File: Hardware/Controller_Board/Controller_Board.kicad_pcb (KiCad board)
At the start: 8 copper layers, 211 parts, among them J103 USB_C_USB2.0, Q1 DMN2400UFB-7, SW1 Reset, U1 TPS82084, U10 FT232H, U11 93LC56B, U12 USB2512B, U14 RJ45, U15 TPD4E02B04, U16 RJ45, U17 RJ45, U18 TPD4E02B04, U19 TPD4E02B04, U2 LT8645S, U20 TPD4E02B04, U21 TPD4E02B04, U22 RJ45, U23 TPD4E02B04, U24 TPD4E02B04, U25 RJ45, U26 TPD4E02B04, U27 TPD4E02B04, U28 RJ45, U29 TPD4E02B04, U3 TPS82084, U30 TPD4E02B04, U31 RJ45, U32 TPD4E02B04, U33 TPD4E02B04, U34 RJ45, U37 RJ45, U39 TPD4E02B04, U4 TPS82084, U5 XT30, U501 TPD4E02B04, U6 XC7A35T-CPG236, U7 IS25LP256D, U8 FT232H, U9 93LC56B, Y1 12MHz, Y2 12MHz, Y3 24MHz, Y301 12MHz

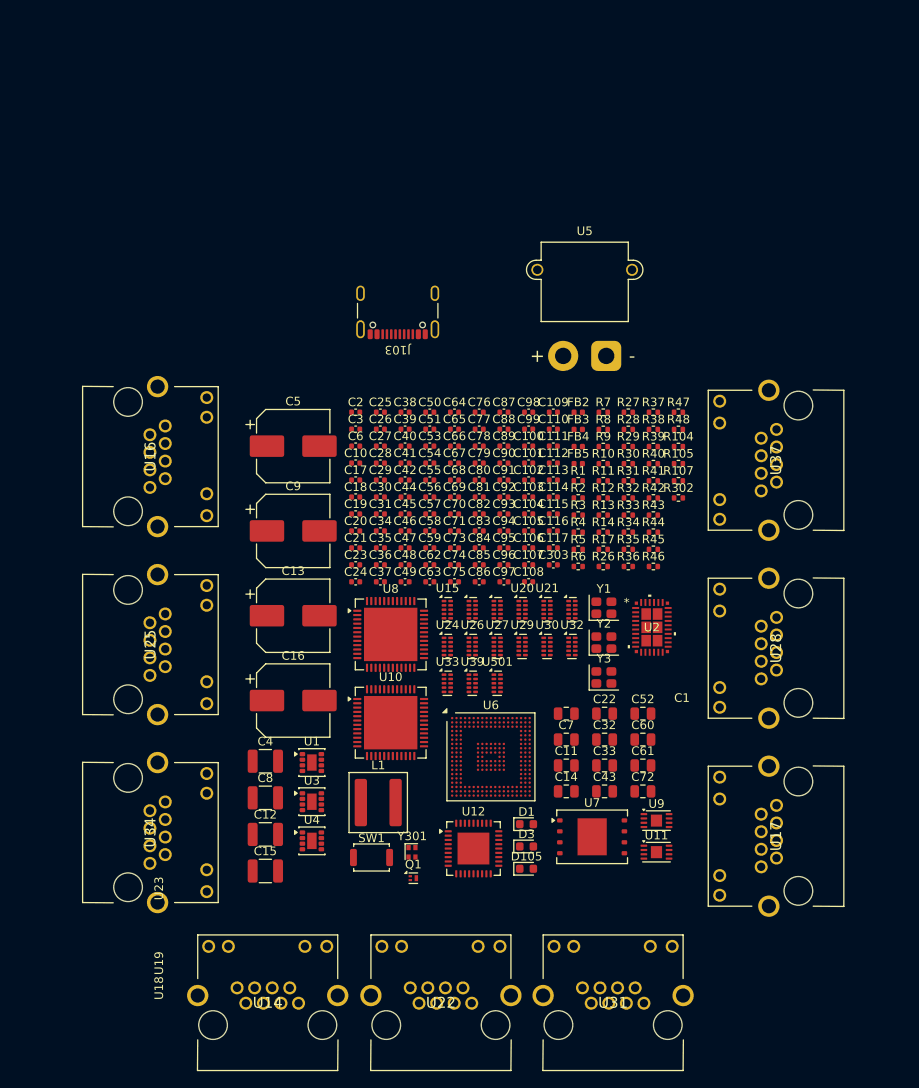
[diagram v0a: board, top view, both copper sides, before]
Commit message: Finished the schematic review
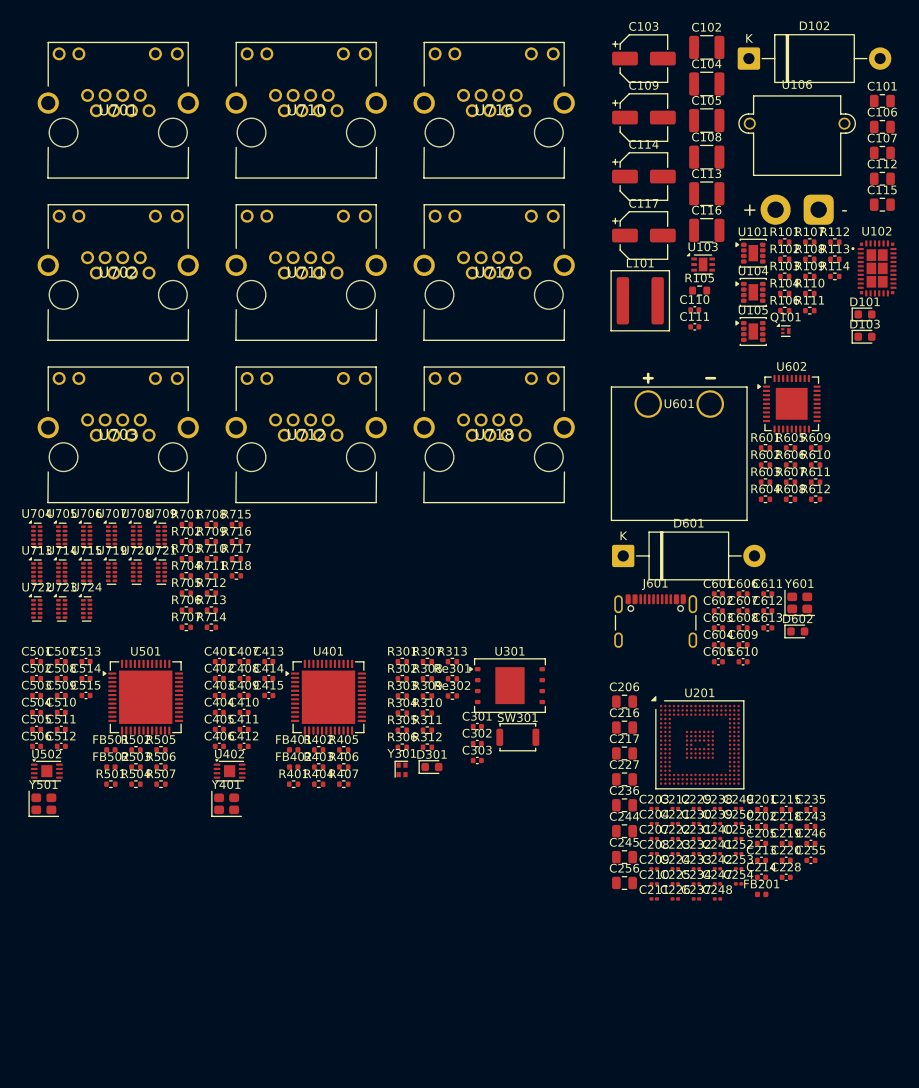
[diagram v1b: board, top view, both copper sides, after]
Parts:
- removed C1, C11, C14, C22, C32, C33, C43, C52, C60, C61, C7, C72: 10u, Capacitor_SMD:C_0805_2012Metric
- removed C10, C17, C19, C20, C23, C24, C25, C26, C27, C28, C37, C38, C39, C40, C41, C42, C45, C46, C47, C48, C49, C50, C53, C54, C55, C56, C57, C58, C63, C64, C65, C66, C67, C68, C69, C70, C73, C76, C77, C78, C79, C80, C81, C82, C84, C86, C87, C91, C92, C93, C94, C95, C96, C97, C99: 100n, Capacitor_SMD:C_0402_1005Metric
- removed C100, C75, C83, C85, C90, C98: 4u7, Capacitor_SMD:C_0402_1005Metric
- removed C12, C15, C4, C8: 22u, Capacitor_SMD:C_1210_3225Metric
- removed C13, C16, C5, C9: 100u, Capacitor_SMD:CP_Elec_8x6.5
- removed C18, C88, C89: 10p, Capacitor_SMD:C_0402_1005Metric
- removed C2, C3: 470n, Capacitor_SMD:C_0402_1005Metric
- removed C21, C29, C30, C31, C34, C35, C36, C44, C51, C59, C62, C71, C74: 1u, Capacitor_SMD:C_0402_1005Metric
- removed C6: 2.2p, Capacitor_SMD:C_0402_1005Metric
- removed D1, D105, D3: LED, LED_SMD:LED_0603_1608Metric
- removed FB2, FB3, FB4, FB5: 600R, Inductor_SMD:L_0402_1005Metric
- removed J103: USB_C_USB2.0, Connector_USB:USB_C_Receptacle_GCT_USB4105-xx-A_16P_TopMnt_Horizontal
- removed L1: 2u2, Inductor_SMD:L_Coilcraft_XAL6030-XXX
- removed Q1: DMN2400UFB-7, Package_DFN_QFN:Diodes_DFN1006-3
- removed R1: 1Meg, Resistor_SMD:R_0402_1005Metric
- removed R10, R2, R7: 499k, Resistor_SMD:R_0402_1005Metric
- removed R11: 156.3k, Resistor_SMD:R_0402_1005Metric
- removed R12, R5, R9: 50k, Resistor_SMD:R_0402_1005Metric
- removed R13: 280R, Resistor_SMD:R_0402_1005Metric
- removed R14, R17: 200R, Resistor_SMD:R_0402_1005Metric
- removed R26, R33, R48: 1k, Resistor_SMD:R_0402_1005Metric
- removed R27, R34, R41: 12k, Resistor_SMD:R_0402_1005Metric
- removed R28, R29, R30, R35, R36, R37: 10k, Resistor_SMD:R_0402_1005Metric
- removed R3: 12.5k, Resistor_SMD:R_0402_1005Metric
- removed R31, R38: 2k2, Resistor_SMD:R_0402_1005Metric
- removed R32, R39, R40: 22R, Resistor_SMD:R_0402_1005Metric
- removed R4: 243k, Resistor_SMD:R_0402_1005Metric
- removed R42, R43, R44, R45, R46, R47: 100k, Resistor_SMD:R_0402_1005Metric
- removed R6: 41.2k, Resistor_SMD:R_0402_1005Metric
- removed R8: 62.5k, Resistor_SMD:R_0402_1005Metric
- removed SW1: Reset, Button_Switch_SMD:SW_Push_SPST_NO_Alps_SKRK
- removed U1, U3, U4: TPS82084, Package_LGA:Texas_SIL0008C_MicroSiP-8-1EP_2.8x3mm_P0.65mm_EP1.1x1.9mm
- removed U10, U8: FT232H, Package_DFN_QFN:QFN-48-1EP_8x8mm_P0.5mm_EP6.2x6.2mm
- removed U11, U9: 93LC56B, Package_DFN_QFN:TDFN-8-1EP_3x2mm_P0.5mm_EP1.3x1.4mm
- removed U12: USB2512B, Package_DFN_QFN:QFN-36-1EP_6x6mm_P0.5mm_EP3.7x3.7mm
- removed U14, U16, U17, U22, U25, U28, U31, U34, U37: RJ45, Custom_VoxLink_Footprints:TE_RJ45
- removed U15, U18, U19, U20, U21, U23, U24, U26, U27, U29, U30, U32, U33, U39: TPD4E02B04, Package_SON:USON-10_2.5x1.0mm_P0.5mm
- removed U2: LT8645S, Custom_VoxLink_Footprints:LT8645S
- removed U5: XT30, Connector_AMASS:AMASS_XT30PW-M_1x02_P2.50mm_Horizontal
- removed U6: XC7A35T-CPG236, Package_BGA:Xilinx_CPG236
- removed U7: IS25LP256D, Package_SON:WSON-8-1EP_8x6mm_P1.27mm_EP3.4x4.3mm
- removed Y1, Y2: 12MHz, Crystal:Crystal_SMD_2520-4Pin_2.5x2.0mm
- removed Y3: 24MHz, Crystal:Crystal_SMD_2520-4Pin_2.5x2.0mm
- added C201: 100n, Capacitor_SMD:C_0402_1005Metric, F.Cu at (160.2, 121.0)
- added C202: 10p, Capacitor_SMD:C_0402_1005Metric, F.Cu at (160.2, 122.9)
- added C203: 100n, Capacitor_SMD:C_0201_0603Metric, F.Cu at (147.8, 120.8)
- added C204: 100n, Capacitor_SMD:C_0201_0603Metric, F.Cu at (147.8, 122.6)
- added C205: 1u, Capacitor_SMD:C_0402_1005Metric, F.Cu at (160.2, 124.9)
- added C206: 10u, Capacitor_SMD:C_0805_2012Metric, F.Cu at (144.3, 108.4)
- added C207: 100n, Capacitor_SMD:C_0201_0603Metric, F.Cu at (147.8, 124.3)
- added C208: 100n, Capacitor_SMD:C_0201_0603Metric, F.Cu at (147.8, 126.1)
- added C209: 100n, Capacitor_SMD:C_0201_0603Metric, F.Cu at (147.8, 127.8)
- added C210: 100n, Capacitor_SMD:C_0201_0603Metric, F.Cu at (147.8, 129.6)
- added C211: 100n, Capacitor_SMD:C_0201_0603Metric, F.Cu at (147.8, 131.3)
- added C212: 100n, Capacitor_SMD:C_0201_0603Metric, F.Cu at (150.2, 120.8)
- added C213: 1u, Capacitor_SMD:C_0402_1005Metric, F.Cu at (160.2, 126.9)
- added C214: 1u, Capacitor_SMD:C_0402_1005Metric, F.Cu at (160.2, 128.8)
- added C215: 1u, Capacitor_SMD:C_0402_1005Metric, F.Cu at (163.1, 121.0)
- added C216: 10u, Capacitor_SMD:C_0805_2012Metric, F.Cu at (144.3, 111.4)
- added C217: 10u, Capacitor_SMD:C_0805_2012Metric, F.Cu at (144.3, 114.5)
- added C218: 1u, Capacitor_SMD:C_0402_1005Metric, F.Cu at (163.1, 122.9)
- added C219: 1u, Capacitor_SMD:C_0402_1005Metric, F.Cu at (163.1, 124.9)
- added C220: 1u, Capacitor_SMD:C_0402_1005Metric, F.Cu at (163.1, 126.9)
- added C221: 100n, Capacitor_SMD:C_0201_0603Metric, F.Cu at (150.2, 122.6)
- added C222: 100n, Capacitor_SMD:C_0201_0603Metric, F.Cu at (150.2, 124.3)
- added C223: 100n, Capacitor_SMD:C_0201_0603Metric, F.Cu at (150.2, 126.1)
- added C224: 100n, Capacitor_SMD:C_0201_0603Metric, F.Cu at (150.2, 127.8)
- added C225: 100n, Capacitor_SMD:C_0201_0603Metric, F.Cu at (150.2, 129.6)
- added C226: 100n, Capacitor_SMD:C_0201_0603Metric, F.Cu at (150.2, 131.3)
- added C227: 10u, Capacitor_SMD:C_0805_2012Metric, F.Cu at (144.3, 117.5)
- added C228: 1u, Capacitor_SMD:C_0402_1005Metric, F.Cu at (163.1, 128.8)
- added C229: 100n, Capacitor_SMD:C_0201_0603Metric, F.Cu at (152.7, 120.8)
- added C230: 100n, Capacitor_SMD:C_0201_0603Metric, F.Cu at (152.7, 122.6)
- added C231: 100n, Capacitor_SMD:C_0201_0603Metric, F.Cu at (152.7, 124.3)
- added C232: 100n, Capacitor_SMD:C_0201_0603Metric, F.Cu at (152.7, 126.1)
- added C233: 100n, Capacitor_SMD:C_0201_0603Metric, F.Cu at (152.7, 127.8)
- added C234: 100n, Capacitor_SMD:C_0201_0603Metric, F.Cu at (152.7, 129.6)
- added C235: 1u, Capacitor_SMD:C_0402_1005Metric, F.Cu at (166.0, 121.0)
- added C236: 10u, Capacitor_SMD:C_0805_2012Metric, F.Cu at (144.3, 120.5)
- added C237: 100n, Capacitor_SMD:C_0201_0603Metric, F.Cu at (152.7, 131.3)
- added C238: 100n, Capacitor_SMD:C_0201_0603Metric, F.Cu at (155.1, 120.8)
- added C239: 100n, Capacitor_SMD:C_0201_0603Metric, F.Cu at (155.1, 122.6)
- added C240: 100n, Capacitor_SMD:C_0201_0603Metric, F.Cu at (155.1, 124.3)
- added C241: 100n, Capacitor_SMD:C_0201_0603Metric, F.Cu at (155.1, 126.1)
- added C242: 100n, Capacitor_SMD:C_0201_0603Metric, F.Cu at (155.1, 127.8)
- added C243: 1u, Capacitor_SMD:C_0402_1005Metric, F.Cu at (166.0, 122.9)
- added C244: 10u, Capacitor_SMD:C_0805_2012Metric, F.Cu at (144.3, 123.5)
- added C245: 10u, Capacitor_SMD:C_0805_2012Metric, F.Cu at (144.3, 126.5)
- added C246: 1u, Capacitor_SMD:C_0402_1005Metric, F.Cu at (166.0, 124.9)
- added C247: 100n, Capacitor_SMD:C_0201_0603Metric, F.Cu at (155.1, 129.6)
- added C248: 100n, Capacitor_SMD:C_0201_0603Metric, F.Cu at (155.1, 131.3)
- added C249: 100n, Capacitor_SMD:C_0201_0603Metric, F.Cu at (157.6, 120.8)
- added C250: 100n, Capacitor_SMD:C_0201_0603Metric, F.Cu at (157.6, 122.6)
- added C251: 100n, Capacitor_SMD:C_0201_0603Metric, F.Cu at (157.6, 124.3)
- added C252: 100n, Capacitor_SMD:C_0201_0603Metric, F.Cu at (157.6, 126.1)
- added C253: 100n, Capacitor_SMD:C_0201_0603Metric, F.Cu at (157.6, 127.8)
- added C254: 100n, Capacitor_SMD:C_0201_0603Metric, F.Cu at (157.6, 129.6)
- added C255: 1u, Capacitor_SMD:C_0402_1005Metric, F.Cu at (166.0, 126.9)
- added C256: 10u, Capacitor_SMD:C_0805_2012Metric, F.Cu at (144.3, 129.5)
- added C301: 1u, Capacitor_SMD:C_0402_1005Metric, F.Cu at (127.2, 111.3)
- added C302: 100n, Capacitor_SMD:C_0402_1005Metric, F.Cu at (127.2, 113.3)
- added C401: 4u7, Capacitor_SMD:C_0402_1005Metric, F.Cu at (97.3, 103.8)
- added C402: 100n, Capacitor_SMD:C_0402_1005Metric, F.Cu at (97.3, 105.8)
- added C403: 100n, Capacitor_SMD:C_0402_1005Metric, F.Cu at (97.3, 107.7)
- added C404: 100n, Capacitor_SMD:C_0402_1005Metric, F.Cu at (97.3, 109.7)
- added C405: 100n, Capacitor_SMD:C_0402_1005Metric, F.Cu at (97.3, 111.7)
- added C406: 100n, Capacitor_SMD:C_0402_1005Metric, F.Cu at (97.3, 113.6)
- added C407: 100n, Capacitor_SMD:C_0402_1005Metric, F.Cu at (100.1, 103.8)
- added C408: 100n, Capacitor_SMD:C_0402_1005Metric, F.Cu at (100.1, 105.8)
- added C409: 4u7, Capacitor_SMD:C_0402_1005Metric, F.Cu at (100.1, 107.7)
- added C410: 100n, Capacitor_SMD:C_0402_1005Metric, F.Cu at (100.1, 109.7)
- added C411: 4u7, Capacitor_SMD:C_0402_1005Metric, F.Cu at (100.1, 111.7)
- added C412: 100n, Capacitor_SMD:C_0402_1005Metric, F.Cu at (100.1, 113.6)
- added C413: 100n, Capacitor_SMD:C_0402_1005Metric, F.Cu at (103.0, 103.8)
- added C414: 10p, Capacitor_SMD:C_0402_1005Metric, F.Cu at (103.0, 105.8)
- added C415: 10p, Capacitor_SMD:C_0402_1005Metric, F.Cu at (103.0, 107.7)
- added C501: 4u7, Capacitor_SMD:C_0402_1005Metric, F.Cu at (76.0, 103.8)
- added C502: 100n, Capacitor_SMD:C_0402_1005Metric, F.Cu at (76.0, 105.8)
- added C503: 100n, Capacitor_SMD:C_0402_1005Metric, F.Cu at (76.0, 107.7)
- added C504: 100n, Capacitor_SMD:C_0402_1005Metric, F.Cu at (76.0, 109.7)
- added C505: 100n, Capacitor_SMD:C_0402_1005Metric, F.Cu at (76.0, 111.7)
- added C506: 100n, Capacitor_SMD:C_0402_1005Metric, F.Cu at (76.0, 113.6)
- added C507: 100n, Capacitor_SMD:C_0402_1005Metric, F.Cu at (78.9, 103.8)
- added C508: 100n, Capacitor_SMD:C_0402_1005Metric, F.Cu at (78.9, 105.8)
- added C509: 4u7, Capacitor_SMD:C_0402_1005Metric, F.Cu at (78.9, 107.7)
- added C510: 100n, Capacitor_SMD:C_0402_1005Metric, F.Cu at (78.9, 109.7)
- added C511: 4u7, Capacitor_SMD:C_0402_1005Metric, F.Cu at (78.9, 111.7)
- added C512: 100n, Capacitor_SMD:C_0402_1005Metric, F.Cu at (78.9, 113.6)
- added C513: 100n, Capacitor_SMD:C_0402_1005Metric, F.Cu at (81.8, 103.8)
- added C514: 10p, Capacitor_SMD:C_0402_1005Metric, F.Cu at (81.8, 105.8)
- added C515: 10p, Capacitor_SMD:C_0402_1005Metric, F.Cu at (81.8, 107.7)
- added C601: 4u7, Capacitor_SMD:C_0402_1005Metric, F.Cu at (155.2, 95.9)
- added C602: 100n, Capacitor_SMD:C_0402_1005Metric, F.Cu at (155.2, 97.9)
- added C603: 100n, Capacitor_SMD:C_0402_1005Metric, F.Cu at (155.2, 99.9)
- added C604: 100n, Capacitor_SMD:C_0402_1005Metric, F.Cu at (155.2, 101.8)
- added C605: 100n, Capacitor_SMD:C_0402_1005Metric, F.Cu at (155.2, 103.8)
- added C606: 100n, Capacitor_SMD:C_0402_1005Metric, F.Cu at (158.1, 95.9)
- added C607: 100n, Capacitor_SMD:C_0402_1005Metric, F.Cu at (158.1, 97.9)
- added C608: 10n, Capacitor_SMD:C_0402_1005Metric, F.Cu at (158.1, 99.9)
- added C609: 100n, Capacitor_SMD:C_0402_1005Metric, F.Cu at (158.1, 101.8)
- added C610: 10n, Capacitor_SMD:C_0402_1005Metric, F.Cu at (158.1, 103.8)
- added C611: 100n, Capacitor_SMD:C_0402_1005Metric, F.Cu at (161.0, 95.9)
- added C612: 10p, Capacitor_SMD:C_0402_1005Metric, F.Cu at (161.0, 97.9)
- added C613: 10p, Capacitor_SMD:C_0402_1005Metric, F.Cu at (161.0, 99.9)
- added D101: LED, LED_SMD:LED_0603_1608Metric, F.Cu at (172.3, 63.5)
- added D102: TVS, Diode_THT:D_DO-201AE_P15.24mm_Horizontal, F.Cu at (158.8, 33.7)
- added D103: TVS/Zener, Diode_SMD:D_0603_1608Metric, F.Cu at (172.3, 66.0)
- added D301: LED, LED_SMD:LED_0603_1608Metric, F.Cu at (122.0, 116.0)
- added D601: TVS, Diode_THT:D_DO-201AE_P15.24mm_Horizontal, F.Cu at (144.2, 91.5)
- added D602: LED, LED_SMD:LED_0603_1608Metric, F.Cu at (164.4, 100.3)
- added FB201: 600R/100MHz, Inductor_SMD:L_0402_1005Metric, F.Cu at (160.3, 130.8)
- added FB401: 600R, Inductor_SMD:L_0402_1005Metric, F.Cu at (105.9, 114.0)
- added FB402: 600R, Inductor_SMD:L_0402_1005Metric, F.Cu at (105.9, 116.0)
- added FB501: 600R, Inductor_SMD:L_0402_1005Metric, F.Cu at (84.7, 114.0)
- added FB502: 600R, Inductor_SMD:L_0402_1005Metric, F.Cu at (84.7, 116.0)
- added J601: USB-C, Connector_USB:USB_C_Receptacle_GCT_USB4105-xx-A_16P_TopMnt_Horizontal, F.Cu at (147.9, 100.2)
- added L101: 2u2, Inductor_SMD:L_Coilcraft_XAL6030-XXX, F.Cu at (146.2, 61.9)
- added Q101: DMN2400UFB-7, Package_DFN_QFN:Diodes_DFN1006-3, F.Cu at (163.1, 65.4)
- added R101: 499k, Resistor_SMD:R_0402_1005Metric, F.Cu at (162.9, 55.1)
- added R102: 12.5k, Resistor_SMD:R_0402_1005Metric, F.Cu at (162.9, 57.0)
- added R103: 50k, Resistor_SMD:R_0402_1005Metric, F.Cu at (162.9, 59.0)
- added R106: 243k, Resistor_SMD:R_0402_1005Metric, F.Cu at (162.9, 63.0)
- added R108: 499k, Resistor_SMD:R_0402_1005Metric, F.Cu at (165.8, 57.0)
- added R109: 62.5k, Resistor_SMD:R_0402_1005Metric, F.Cu at (165.8, 59.0)
- added R110: 50k, Resistor_SMD:R_0402_1005Metric, F.Cu at (165.8, 61.0)
- added R111: 280R, Resistor_SMD:R_0402_1005Metric, F.Cu at (165.8, 63.0)
- added R112: 499k, Resistor_SMD:R_0402_1005Metric, F.Cu at (168.8, 55.1)
- added R113: 156.3k, Resistor_SMD:R_0402_1005Metric, F.Cu at (168.8, 57.0)
- added R114: 50k, Resistor_SMD:R_0402_1005Metric, F.Cu at (168.8, 59.0)
- added R301: 200R, Resistor_SMD:R_0402_1005Metric, F.Cu at (118.5, 103.8)
- added R303: 200R, Resistor_SMD:R_0402_1005Metric, F.Cu at (118.5, 107.8)
- added R304: 1k, Resistor_SMD:R_0402_1005Metric, F.Cu at (118.5, 109.8)
- added R305: 4.7k, Resistor_SMD:R_0402_1005Metric, F.Cu at (118.5, 111.8)
- added R306: 4.7k, Resistor_SMD:R_0402_1005Metric, F.Cu at (118.5, 113.7)
- added R307: 4.7k, Resistor_SMD:R_0402_1005Metric, F.Cu at (121.4, 103.8)
- added R308: 100R, Resistor_SMD:R_0402_1005Metric, F.Cu at (121.4, 105.8)
- added R309: 100R, Resistor_SMD:R_0402_1005Metric, F.Cu at (121.4, 107.8)
- added R310: 100R, Resistor_SMD:R_0402_1005Metric, F.Cu at (121.4, 109.8)
- added R311: 100R, Resistor_SMD:R_0402_1005Metric, F.Cu at (121.4, 111.8)
- added R312: 100R, Resistor_SMD:R_0402_1005Metric, F.Cu at (121.4, 113.7)
- added R313: 22R, Resistor_SMD:R_0402_1005Metric, F.Cu at (124.3, 103.8)
- added R401: 1k, Resistor_SMD:R_0402_1005Metric, F.Cu at (105.9, 118.0)
- added R402: 12k, Resistor_SMD:R_0402_1005Metric, F.Cu at (108.8, 114.0)
- added R403: 10k, Resistor_SMD:R_0402_1005Metric, F.Cu at (108.8, 116.0)
- added R404: 10k, Resistor_SMD:R_0402_1005Metric, F.Cu at (108.8, 118.0)
- added R405: 10k, Resistor_SMD:R_0402_1005Metric, F.Cu at (111.7, 114.0)
- added R406: 2k2, Resistor_SMD:R_0402_1005Metric, F.Cu at (111.7, 116.0)
- added R407: 22R, Resistor_SMD:R_0402_1005Metric, F.Cu at (111.7, 118.0)
- added R501: 1k, Resistor_SMD:R_0402_1005Metric, F.Cu at (84.7, 118.0)
- added R502: 12k, Resistor_SMD:R_0402_1005Metric, F.Cu at (87.6, 114.0)
- added R503: 10k, Resistor_SMD:R_0402_1005Metric, F.Cu at (87.6, 116.0)
- added R504: 10k, Resistor_SMD:R_0402_1005Metric, F.Cu at (87.6, 118.0)
- added R505: 10k, Resistor_SMD:R_0402_1005Metric, F.Cu at (90.5, 114.0)
- added R506: 2k2, Resistor_SMD:R_0402_1005Metric, F.Cu at (90.5, 116.0)
- added R507: 22R, Resistor_SMD:R_0402_1005Metric, F.Cu at (90.5, 118.0)
- added R601: 1k, Resistor_SMD:R_0402_1005Metric, F.Cu at (160.7, 79.0)
- added R602: 5k1, Resistor_SMD:R_0402_1005Metric, F.Cu at (160.7, 81.0)
- added R603: 5k1, Resistor_SMD:R_0402_1005Metric, F.Cu at (160.7, 82.9)
- added R604: 1k, Resistor_SMD:R_0402_1005Metric, F.Cu at (160.7, 84.9)
- added R605: 12k, Resistor_SMD:R_0402_1005Metric, F.Cu at (163.6, 79.0)
- added R606: 100k, Resistor_SMD:R_0402_1005Metric, F.Cu at (163.6, 81.0)
- added R607: 100k, Resistor_SMD:R_0402_1005Metric, F.Cu at (163.6, 82.9)
- added R608: 100k, Resistor_SMD:R_0402_1005Metric, F.Cu at (163.6, 84.9)
- added R609: 100k, Resistor_SMD:R_0402_1005Metric, F.Cu at (166.5, 79.0)
- added R610: 100k, Resistor_SMD:R_0402_1005Metric, F.Cu at (166.5, 81.0)
- added R611: 22R, Resistor_SMD:R_0402_1005Metric, F.Cu at (166.5, 82.9)
- added R612: 100k, Resistor_SMD:R_0402_1005Metric, F.Cu at (166.5, 84.9)
- added R701: 1k, Resistor_SMD:R_0402_1005Metric, F.Cu at (93.4, 87.9)
- added R702: 1k, Resistor_SMD:R_0402_1005Metric, F.Cu at (93.4, 89.8)
- added R703: 1k, Resistor_SMD:R_0402_1005Metric, F.Cu at (93.4, 91.8)
- added R704: 1k, Resistor_SMD:R_0402_1005Metric, F.Cu at (93.4, 93.8)
- added R705: 1k, Resistor_SMD:R_0402_1005Metric, F.Cu at (93.4, 95.8)
- added R706: 1k, Resistor_SMD:R_0402_1005Metric, F.Cu at (93.4, 97.8)
- added R707: 1k, Resistor_SMD:R_0402_1005Metric, F.Cu at (93.4, 99.8)
- added R708: 1k, Resistor_SMD:R_0402_1005Metric, F.Cu at (96.3, 87.9)
- added R709: 1k, Resistor_SMD:R_0402_1005Metric, F.Cu at (96.3, 89.8)
- added R710: 1k, Resistor_SMD:R_0402_1005Metric, F.Cu at (96.3, 91.8)
- added R711: 1k, Resistor_SMD:R_0402_1005Metric, F.Cu at (96.3, 93.8)
- added R712: 1k, Resistor_SMD:R_0402_1005Metric, F.Cu at (96.3, 95.8)
- added R713: 1k, Resistor_SMD:R_0402_1005Metric, F.Cu at (96.3, 97.8)
- added R714: 1k, Resistor_SMD:R_0402_1005Metric, F.Cu at (96.3, 99.8)
- added R715: 1k, Resistor_SMD:R_0402_1005Metric, F.Cu at (99.2, 87.9)
- added R716: 1k, Resistor_SMD:R_0402_1005Metric, F.Cu at (99.2, 89.8)
- added R717: 1k, Resistor_SMD:R_0402_1005Metric, F.Cu at (99.2, 91.8)
- added R718: 1k, Resistor_SMD:R_0402_1005Metric, F.Cu at (99.2, 93.8)
- added Re301: 1k, Resistor_SMD:R_0402_1005Metric, F.Cu at (124.3, 105.8)
- added Re302: 1k, Resistor_SMD:R_0402_1005Metric, F.Cu at (124.3, 107.8)
- added SW301: Reset, Button_Switch_SMD:SW_Push_SPST_NO_Alps_SKRK, F.Cu at (131.9, 112.6)
- added U101: TPS82084, Package_LGA:Texas_SIL0008C_MicroSiP-8-1EP_2.8x3mm_P0.65mm_EP1.1x1.9mm, F.Cu at (159.3, 56.3)
- added U102: LT8645S, Custom_VoxLink_Footprints:LQFN-32-6EP_6x4mm_P0.5mm_EP1.355x1.125mm, F.Cu at (173.6, 58.1)
- added U103: TDS5311P, Package_DFN_QFN:DFN-6-1EP_2x2mm_P0.65mm_EP1x1.6mm, F.Cu at (153.4, 57.7)
- added U104: TPS82084, Package_LGA:Texas_SIL0008C_MicroSiP-8-1EP_2.8x3mm_P0.65mm_EP1.1x1.9mm, F.Cu at (159.3, 60.9)
- added U105: TPS82084, Package_LGA:Texas_SIL0008C_MicroSiP-8-1EP_2.8x3mm_P0.65mm_EP1.1x1.9mm, F.Cu at (159.3, 65.4)
- added U106: XT30, Connector_AMASS:AMASS_XT30PW-M_1x02_P2.50mm_Horizontal, F.Cu at (166.9, 51.3)
- added U201: XC7A35T-CPG236, Package_BGA:Xilinx_CPG236, F.Cu at (153.1, 113.5)
- added U301: IS25LP256D, Package_SON:WSON-8-1EP_8x6mm_P1.27mm_EP3.4x4.3mm, F.Cu at (131.0, 106.6)
- added U401: FT232H, Package_DFN_QFN:QFN-48-1EP_8x8mm_P0.5mm_EP6.2x6.2mm, F.Cu at (109.9, 107.9)
- added U402: 93LC56B, Package_DFN_QFN:TDFN-8-1EP_3x2mm_P0.5mm_EP1.3x1.4mm, F.Cu at (98.5, 116.5)
- added U502: 93LC56B, Package_DFN_QFN:TDFN-8-1EP_3x2mm_P0.5mm_EP1.3x1.4mm, F.Cu at (77.2, 116.5)
- added U601: ESD122, Amass_XT60:CONN_XT60PW-M_AMA, F.Cu at (147.1, 73.9)
- added U602: USB2512B, Package_DFN_QFN:QFN-36-1EP_6x6mm_P0.5mm_EP3.7x3.7mm, F.Cu at (163.8, 73.8)
- added U701: RJ45, Custom_VoxLink_Footprints:TE_RJ45, F.Cu at (85.5, 42.3)
- added U702: RJ45, Custom_VoxLink_Footprints:TE_RJ45, F.Cu at (85.5, 61.2)
- added U703: RJ45, Custom_VoxLink_Footprints:TE_RJ45, F.Cu at (85.5, 80.0)
- added U704: TPD4E02B04, Package_SON:USON-10_2.5x1.0mm_P0.5mm, F.Cu at (76.1, 89.1)
- added U705: TPD4E02B04, Package_SON:USON-10_2.5x1.0mm_P0.5mm, F.Cu at (79.0, 89.1)
- added U706: TPD4E02B04, Package_SON:USON-10_2.5x1.0mm_P0.5mm, F.Cu at (81.8, 89.1)
- added U707: TPD4E02B04, Package_SON:USON-10_2.5x1.0mm_P0.5mm, F.Cu at (84.7, 89.1)
- added U708: TPD4E02B04, Package_SON:USON-10_2.5x1.0mm_P0.5mm, F.Cu at (87.6, 89.1)
- added U709: TPD4E02B04, Package_SON:USON-10_2.5x1.0mm_P0.5mm, F.Cu at (90.5, 89.1)
- added U710: RJ45, Custom_VoxLink_Footprints:TE_RJ45, F.Cu at (107.4, 42.3)
- added U711: RJ45, Custom_VoxLink_Footprints:TE_RJ45, F.Cu at (107.4, 61.2)
- added U712: RJ45, Custom_VoxLink_Footprints:TE_RJ45, F.Cu at (107.4, 80.0)
- added U713: TPD4E02B04, Package_SON:USON-10_2.5x1.0mm_P0.5mm, F.Cu at (76.1, 93.4)
- added U714: TPD4E02B04, Package_SON:USON-10_2.5x1.0mm_P0.5mm, F.Cu at (79.0, 93.4)
- added U715: TPD4E02B04, Package_SON:USON-10_2.5x1.0mm_P0.5mm, F.Cu at (81.8, 93.4)
- added U716: RJ45, Custom_VoxLink_Footprints:TE_RJ45, F.Cu at (129.2, 42.3)
- added U717: RJ45, Custom_VoxLink_Footprints:TE_RJ45, F.Cu at (129.2, 61.2)
- added U718: RJ45, Custom_VoxLink_Footprints:TE_RJ45, F.Cu at (129.2, 80.0)
- added U719: TPD4E02B04, Package_SON:USON-10_2.5x1.0mm_P0.5mm, F.Cu at (84.7, 93.4)
- added U720: TPD4E02B04, Package_SON:USON-10_2.5x1.0mm_P0.5mm, F.Cu at (87.6, 93.4)
- added U721: TPD4E02B04, Package_SON:USON-10_2.5x1.0mm_P0.5mm, F.Cu at (90.5, 93.4)
- added U722: TPD4E02B04, Package_SON:USON-10_2.5x1.0mm_P0.5mm, F.Cu at (76.1, 97.7)
- added U723: TPD4E02B04, Package_SON:USON-10_2.5x1.0mm_P0.5mm, F.Cu at (79.0, 97.7)
- added U724: TPD4E02B04, Package_SON:USON-10_2.5x1.0mm_P0.5mm, F.Cu at (81.8, 97.7)
- added Y401: 12MHz, Crystal:Crystal_SMD_2520-4Pin_2.5x2.0mm, F.Cu at (98.1, 120.3)
- added Y501: 12MHz, Crystal:Crystal_SMD_2520-4Pin_2.5x2.0mm, F.Cu at (76.9, 120.3)
- added Y601: 24MHz, Crystal:Crystal_SMD_2520-4Pin_2.5x2.0mm, F.Cu at (164.7, 97.0)
- C101, C112, C115: value 100n -> 10u; footprint Capacitor_SMD:C_0402_1005Metric -> Capacitor_SMD:C_0805_2012Metric
- C102, C108, C113: value 100n -> 22u; footprint Capacitor_SMD:C_0402_1005Metric -> Capacitor_SMD:C_1210_3225Metric
- C103: value 10p -> 100u; footprint Capacitor_SMD:C_0402_1005Metric -> Capacitor_SMD:CP_Elec_5x5.9
- C104, C105: value 10p -> 10u; footprint Capacitor_SMD:C_0402_1005Metric -> Capacitor_SMD:C_1210_3225Metric
- C106: value 10p -> 100n; footprint Capacitor_SMD:C_0402_1005Metric -> Capacitor_SMD:C_0805_2012Metric
- C107: value 4u7 -> 100n; footprint Capacitor_SMD:C_0402_1005Metric -> Capacitor_SMD:C_0805_2012Metric
- C109, C117: value 100n -> 100u; footprint Capacitor_SMD:C_0402_1005Metric -> Capacitor_SMD:CP_Elec_5x5.9
- C110: value 100n -> 2.2p
- C111: value 100n -> 10n
- C114: value 10n -> 100u; footprint Capacitor_SMD:C_0402_1005Metric -> Capacitor_SMD:CP_Elec_5x5.9
- C116: value 10n -> 22u; footprint Capacitor_SMD:C_0402_1005Metric -> Capacitor_SMD:C_1210_3225Metric
- R104: value 5k1 -> 1Meg
- R105: value 5k1 -> 1R; footprint Resistor_SMD:R_0402_1005Metric -> Resistor_SMD:R_0603_1608Metric
- R107: value 1k -> 41.2k
- R302: value 22R -> 4.7k
- U501: value TPD4E02B04 -> FT232H; footprint Package_SON:USON-10_2.5x1.0mm_P0.5mm -> Package_DFN_QFN:QFN-48-1EP_8x8mm_P0.5mm_EP6.2x6.2mm
- moved C106 63.9 mm to (174.3, 41.7)
- moved C107 63.1 mm to (174.3, 44.7)
- moved C101 58.8 mm to (174.3, 38.7)
- moved C102 54.3 mm to (153.9, 32.4)
- moved C104 54.1 mm to (153.9, 36.7)
- moved C108 53.5 mm to (153.9, 45.2)
- moved C103 52.7 mm to (146.6, 33.7)
- moved C115 52.5 mm to (174.3, 50.7)
- moved C105 52.0 mm to (153.9, 40.9)
- moved C112 50.5 mm to (174.3, 47.7)
- moved U501 40.9 mm to (88.7, 107.9)
- moved C116 39.2 mm to (153.9, 53.7)
- moved C114 38.7 mm to (146.6, 47.4)
- moved R302 38.3 mm to (118.5, 105.8)
- moved C117 37.8 mm to (146.6, 54.3)
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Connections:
- C101 pad 1: +3V3_VPLL -> +5V
- C102 pad 1: +3V3 -> +1V0
- C103 pad 1: /Serial/OSC_IN -> +1V0
- C104 pad 1: Net-(C104-Pad1) -> VIN
- C104 pad 2: GND -> Net-(C104-Pad2)
- C105 pad 1: /USB/OSC_IN -> VIN
- C106 pad 1: Net-(C106-Pad1) -> VIN
- C107 pad 1: +3V3 -> VIN
- C108 pad 1: +3V3 -> +5V
- C109 pad 1: +3V3 -> +5V
- C110 pad 1: +3V3 -> +5V
- C110 pad 2: GND -> /Power/FB_5V0
- C111 pad 1: +3V3 -> /Power/TR/SS
- C112 pad 1: +3V3 -> +5V
- C113 pad 1: +3V3 -> +1V8
- C114 pad 1: Net-(U12-PLLFILT) -> +1V8
- C115 pad 1: Net-(U12-PLLFILT) -> +5V
- C116 pad 1: Net-(U12-CRFILT) -> +3V3
- C117 pad 1: Net-(U12-CRFILT) -> +3V3
- C303 pad 1: VCCIO2 -> +3V3
- R104 pad 1: GND -> +5V
- R104 pad 2: Net-(J103-CC1) -> /Power/FB_5V0
- R105 pad 1: GND -> Net-(C104-Pad2)
- R105 pad 2: Net-(J103-CC2) -> GND
- R107 pad 2: VBUS -> GND
- R302 pad 1: 12MHZ_CLK -> +3V3
- R302 pad 2: /FPGA_Config/OSC_OUT -> Net-(U201B-CFGBVS_0)
- U501 pad 1: /Connectivity/P1_TX_N -> /Serial/OSC_IN
- U501 pad 10: /Connectivity/P1_TX_N -> GND
- U501 pad 2: /Connectivity/P1_TX_P -> /Serial/OSC_OUT
- U501 pad 3: GND -> +3V3_VPHY
- U501 pad 4: /Connectivity/P1_CLK_N -> GND
- U501 pad 5: /Connectivity/P1_CLK_P -> Net-(U501-REF)
- U501 pad 6: /Connectivity/P1_CLK_P -> SERIAL_D-
- U501 pad 7: /Connectivity/P1_CLK_N -> SERIAL_D+
- U501 pad 8: GND -> +3V3_VPLL
- U501 pad 9: /Connectivity/P1_TX_P -> GND
- Y301 pad 1: VCCIO2 -> +3V3
- Y301 pad 4: VCCIO2 -> +3V3
